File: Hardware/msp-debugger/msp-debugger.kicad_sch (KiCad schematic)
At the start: 22 parts, among them J1 USB_B_Micro, J2 Conn_02x10, J3 Conn_02x10, J4 Conn_01x04_Pin, SW1 222ADVBA, SW2 222ADVBA, SW3 222ADVBA, SW4 222ADVBA, SW5 222ADVBA, U1 MSP430G2553IN20, U3 BA033CC0FP-E2, U4 FT230XS-R

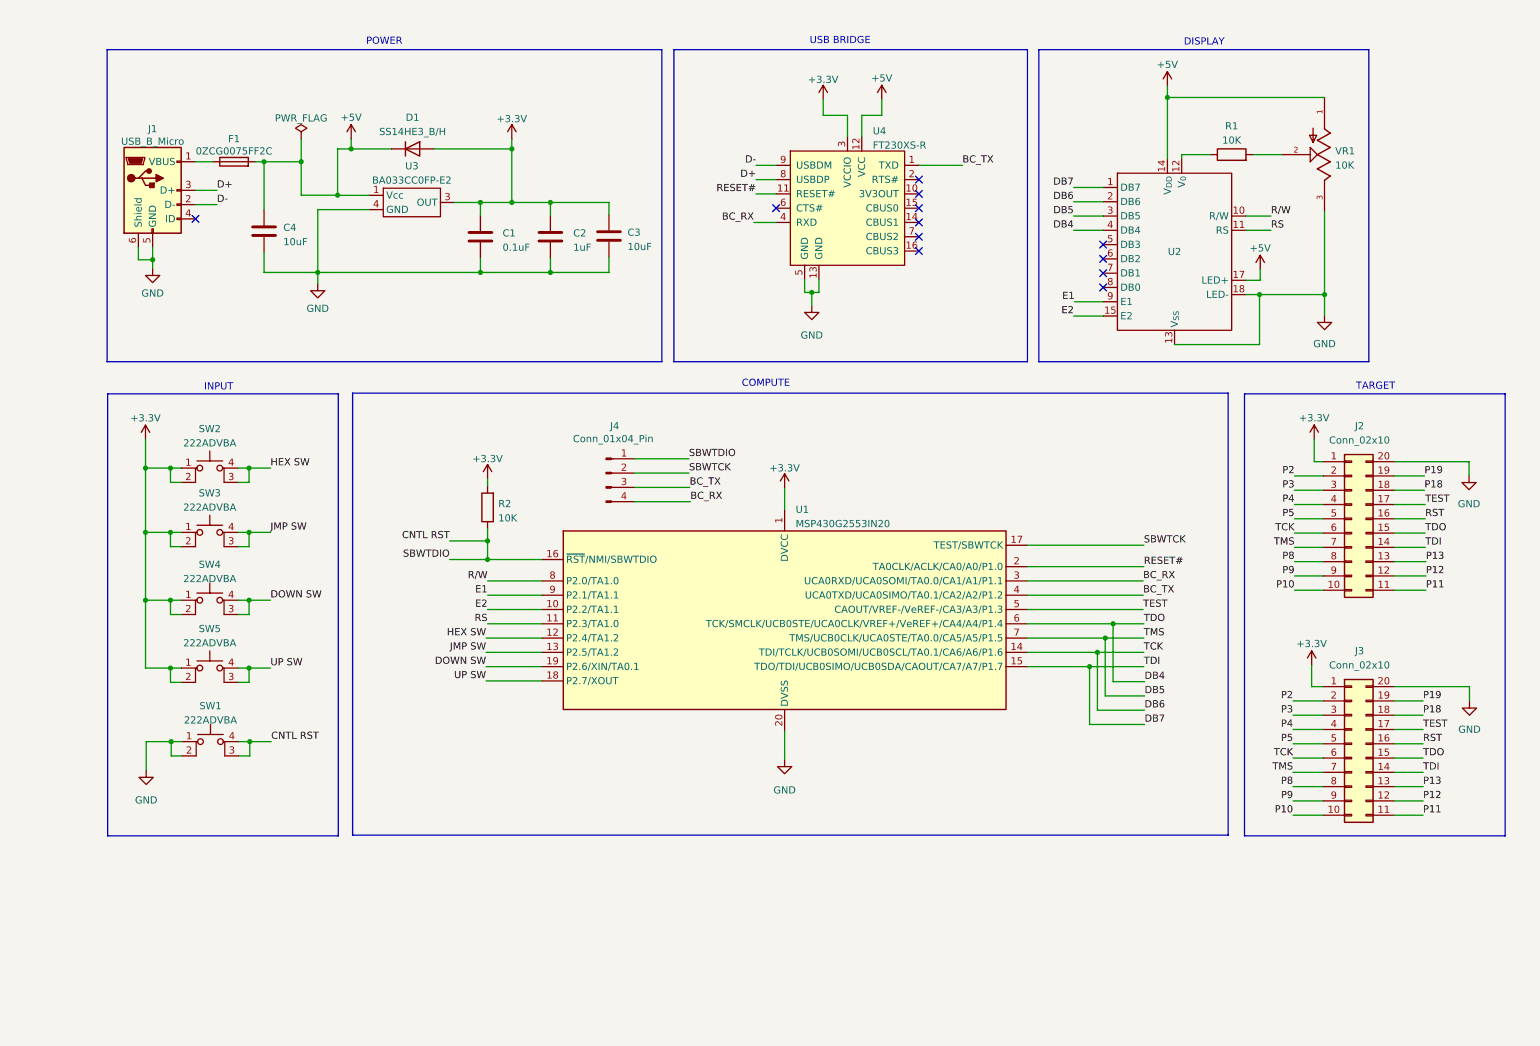
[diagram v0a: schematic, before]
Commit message: fix hardware issues and route small pcb
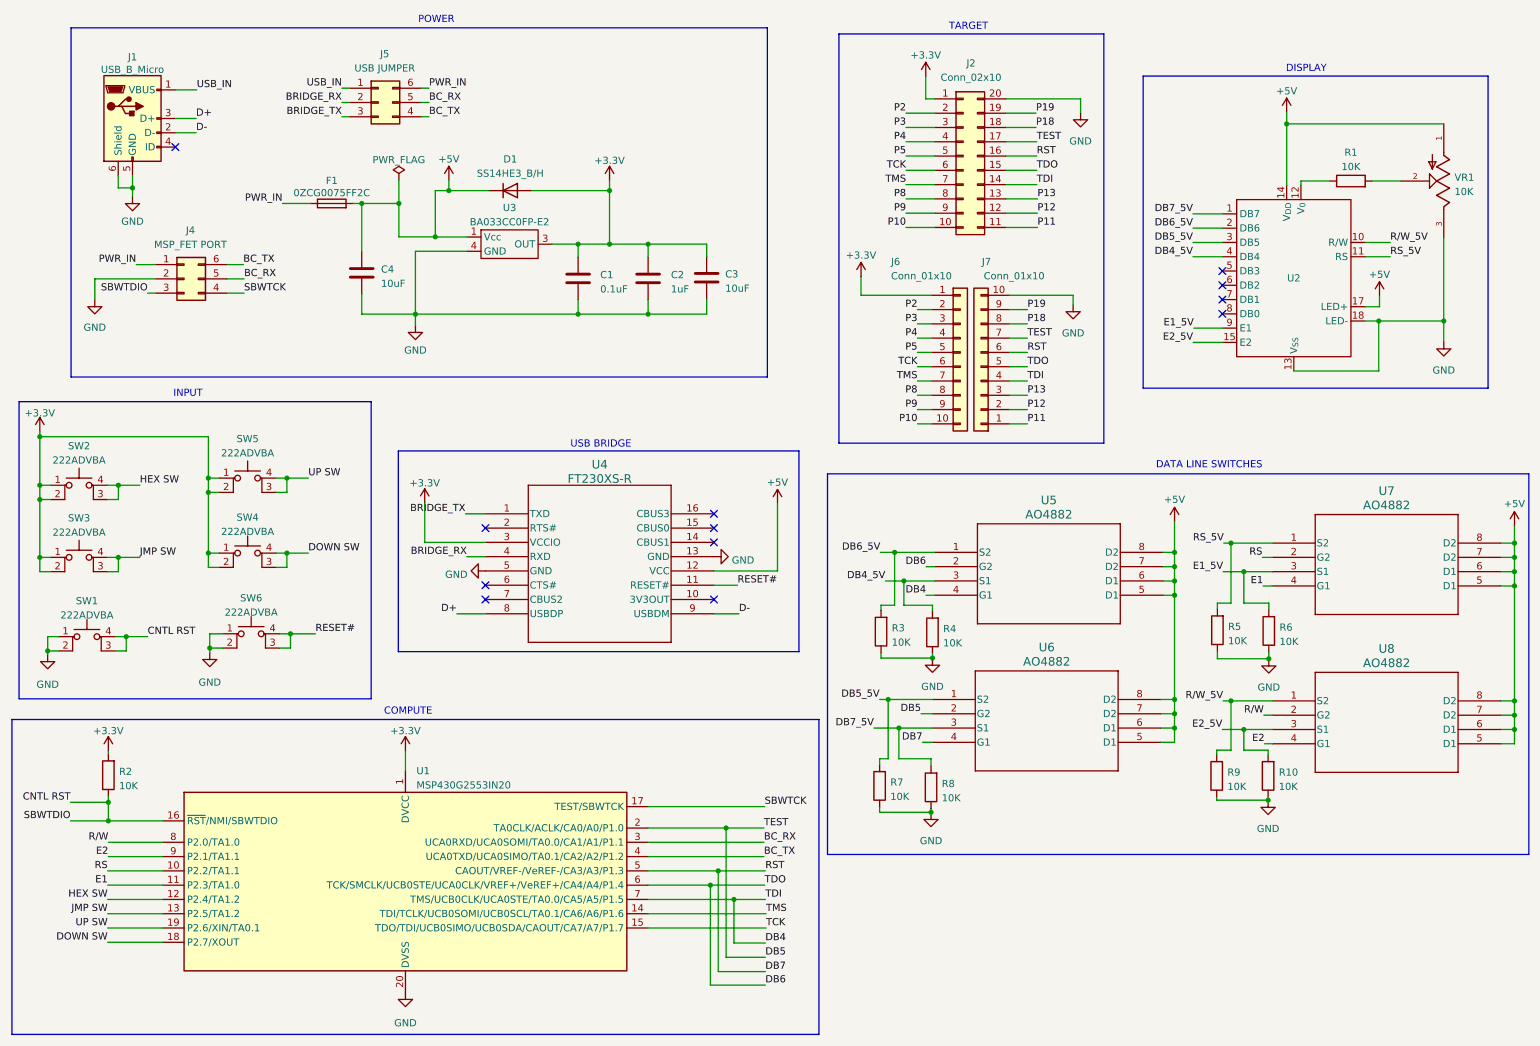
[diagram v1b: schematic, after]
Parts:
- removed J3: Conn_02x10, Connector_PinHeader_2.54mm:PinHeader_2x10_P2.54mm_Vertical, symbol Connector_Generic:Conn_02x10_Counter_Clockwise
- removed J4: Conn_01x04_Pin, Connector_PinHeader_2.54mm:PinHeader_1x04_P2.54mm_Vertical, symbol Connector:Conn_01x04_Pin
- removed U4: FT230XS-R, digikey-footprints:SOIC-16_W3.90mm, symbol dk_Interface-Controllers:FT230XS-R
- added J4: MSP_FET PORT, Connector_PinHeader_2.54mm:PinHeader_2x03_P2.54mm_Vertical, symbol Connector_Generic:Conn_02x03_Counter_Clockwise
- added J5: USB JUMPER, Connector_PinHeader_2.54mm:PinHeader_2x03_P2.54mm_Vertical, symbol Connector_Generic:Conn_02x03_Counter_Clockwise
- added J6, J7: Conn_01x10, Connector_PinHeader_2.54mm:PinHeader_1x10_P2.54mm_Vertical, symbol Connector_Generic:Conn_01x10
- added R10, R3, R4, R5, R6, R7, R8, R9: 10K, Capacitor_SMD:C_0805_2012Metric, symbol Device:R
- added SW6: 222ADVBA, buttons:SW_222ADVBA, symbol Switch:SW_MEC_5E
- added U4: FT230XS-R, SOIC_30XS-R_FTD, symbol ft230xs-r:FT230XS-R
- added U5, U6, U7, U8: AO4882, SO-8_AOS, symbol ao4882:AO4882
- J1: footprint Connector_USB:USB_Micro-B_Amphenol_10118194_Horizontal -> Connector_PinHeader_2.54mm:PinHeader_1x05_P2.54mm_Vertical
- U2: footprint project:NHD-0440AZ-FL-YBW -> Connector_PinHeader_2.54mm:PinHeader_2x09_P2.54mm_Vertical
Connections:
- net RST is gone; now on net DB7: J2.16 (Pin_16)
- net +3.3V: now also J6.1 (Pin_1), U4.3 (VCCIO)
- net +5V: now also U4.12 (VCC), U5.5 (D1), U5.6 (D1), U5.7 (D2), U5.8 (D2), U6.5 (D1), U6.6 (D1), U6.7 (D2), U6.8 (D2), U7.5 (D1), U7.6 (D1), U7.7 (D2), U7.8 (D2), U8.5 (D1), U8.6 (D1), U8.7 (D2), U8.8 (D2)
- net BC_RX: now also J4.5 (Pin_5), J5.5 (Pin_5)
- net BC_TX: now also J4.6 (Pin_6), J5.4 (Pin_4)
- net CNTL RST: now also J4.3 (Pin_3)
- net D+: now also U4.8 (USBDP)
- net D-: now also U4.9 (USBDM)
- net DB4: now also J2.14 (Pin_14), U1.7 (TMS/UCB0CLK/UCA0STE/TA0.0/CA5/A5/P1.5), J7.4 (Pin_4), U5.4 (G1); no longer J2.15 (Pin_15), U1.6 (TCK/SMCLK/UCB0STE/UCA0CLK/VREF+/VeREF+/CA4/A4/P1.4), U2.4 (DB4)
- net DB5: now also J2.17 (Pin_17), U1.2 (TA0CLK/ACLK/CA0/A0/P1.0), J7.7 (Pin_7), U6.2 (G2); no longer J2.7 (Pin_7), U1.7 (TMS/UCB0CLK/UCA0STE/TA0.0/CA5/A5/P1.5), U2.3 (DB5)
- net DB6: now also J2.15 (Pin_15), U1.6 (TCK/SMCLK/UCB0STE/UCA0CLK/VREF+/VeREF+/CA4/A4/P1.4), J7.5 (Pin_5), U5.2 (G2); no longer J2.6 (Pin_6), U1.14 (TDI/TCLK/UCB0SOMI/UCB0SCL/TA0.1/CA6/A6/P1.6), U2.2 (DB6)
- net DB7: now also U1.5 (CAOUT/VREF-/VeREF-/CA3/A3/P1.3), J7.6 (Pin_6), U6.4 (G1); no longer J2.14 (Pin_14), U1.15 (TDO/TDI/UCB0SIMO/UCB0SDA/CAOUT/CA7/A7/P1.7), U2.1 (DB7)
- net DOWN SW: now also U1.18 (P2.7/XOUT); no longer U1.19 (P2.6/XIN/TA0.1)
- net E1: now also U1.11 (P2.3/TA1.0), U7.4 (G1); no longer U1.9 (P2.1/TA1.1), U2.9 (E1)
- net E2: now also U1.9 (P2.1/TA1.1), U8.4 (G1); no longer U1.10 (P2.2/TA1.1), U2.15 (E2)
- net GND: now also J4.2 (Pin_2), J7.10 (Pin_10), R10.1, R3.1, R4.1, R5.1, R6.1, R7.1, R8.1, R9.1, SW6.1, SW6.2, U4.13 (GND), U4.5 (GND)
- net P10: now also J6.10 (Pin_10)
- net P11: now also J7.1 (Pin_1)
- net P12: now also J7.2 (Pin_2)
- net P13: now also J7.3 (Pin_3)
- net P18: now also J7.8 (Pin_8)
- net P19: now also J7.9 (Pin_9)
- net P2: now also J6.2 (Pin_2)
- net P3: now also J6.3 (Pin_3)
- net P4: now also J6.4 (Pin_4)
- net P5: now also J6.5 (Pin_5)
- net P8: now also J6.8 (Pin_8)
- net P9: now also J6.9 (Pin_9)
- net RESET#: now also SW6.3 (K), SW6.4 (A), U4.11 (RESET#); no longer U1.2 (TA0CLK/ACLK/CA0/A0/P1.0)
- net RS: now also U1.10 (P2.2/TA1.1), U7.2 (G2); no longer U1.11 (P2.3/TA1.0), U2.11 (RS)
- net R/W: now also U8.2 (G2); no longer U2.10 (R/W)
- net SBWTCK: now also J4.4 (Pin_4)
- net UP SW: now also U1.19 (P2.6/XIN/TA0.1); no longer U1.18 (P2.7/XOUT)
- net PWR_IN: now reaches F1.1
- net PWR_IN: now also J4.1 (Pin_1), J5.6 (Pin_6); no longer J1.1 (VBUS)
- removed net TEST: J2.17 (Pin_17), U1.5 (CAOUT/VREF-/VeREF-/CA3/A3/P1.3)
- new net BRIDGE_RX: J5.2 (Pin_2), U4.4 (RXD)
- new net BRIDGE_TX: J5.3 (Pin_3), U4.1 (TXD)
- new net DB4_5V: R4.2, U2.4 (DB4), U5.3 (S1)
- new net DB5_5V: R7.2, U2.3 (DB5), U6.1 (S2)
- new net DB6_5V: R3.2, U2.2 (DB6), U5.1 (S2)
- new net DB7_5V: R8.2, U2.1 (DB7), U6.3 (S1)
- new net E1_5V: R6.2, U2.9 (E1), U7.3 (S1)
- new net E2_5V: R10.2, U2.15 (E2), U8.3 (S1)
- new net RS_5V: R5.2, U2.11 (RS), U7.1 (S2)
- new net R/W_5V: R9.2, U2.10 (R/W), U8.1 (S2)
- new net TCK: J2.6 (Pin_6), J6.6 (Pin_6), U1.15 (TDO/TDI/UCB0SIMO/UCB0SDA/CAOUT/CA7/A7/P1.7)
- new net TMS: J2.7 (Pin_7), J6.7 (Pin_7), U1.14 (TDI/TCLK/UCB0SOMI/UCB0SCL/TA0.1/CA6/A6/P1.6)
- new net USB_IN: J1.1 (VBUS), J5.1 (Pin_1)
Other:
- note added: "DATA LINE SWITCHES"
- moved on the sheet: C1, C2, C3, C4, D1, F1, J1, J2, R1, R2, SW1, SW2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
